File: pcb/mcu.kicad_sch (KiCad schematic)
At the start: 35 parts, among them J1 XF2M-1415-1A, SW1 EVQ-Q2B02W, SW2 EVQ-Q2B02W, U1 ESP32-S3-WROOM-1-N8R2

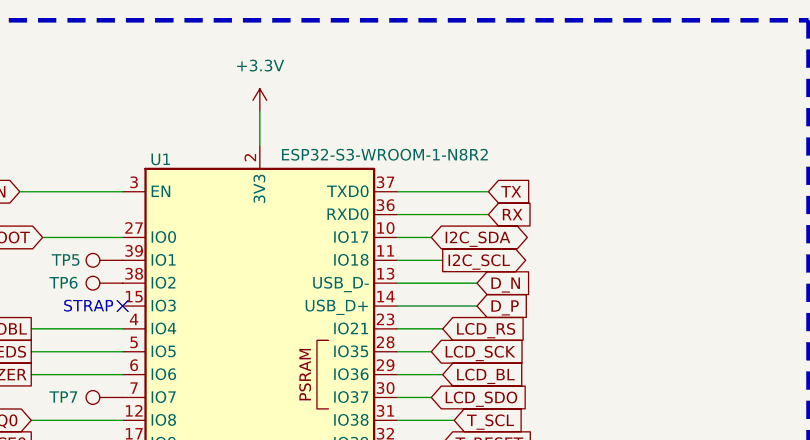
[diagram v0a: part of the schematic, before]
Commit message: Minor updates to ESP part number/footprint
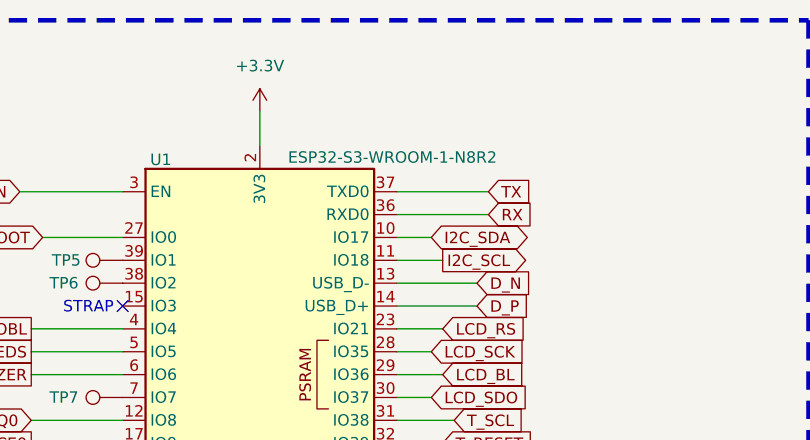
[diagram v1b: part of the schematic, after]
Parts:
- U1: symbol RF_Module:ESP32-S3-WROOM-1 -> CRG Makes:ESP32-S3-WROOM-1-N8R2
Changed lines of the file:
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@@
 	)
 	(symbol
-		(lib_id "RF_Module:ESP32-S3-WROOM-1")
+		(lib_id "CRG Makes:ESP32-S3-WROOM-1-N8R2")
 		(at 73.66 58.42 0)
 		(unit 1)
@@
 		)
 		(property "Value" "ESP32-S3-WROOM-1-N8R2"
-			(at 75.946 31.496 0)
+			(at 88.392 31.75 0)
 			(effects
 				(font
 					(size 1.27 1.27)
 				)
-				(justify left)
 			)
 		)
 		(property "Footprint" "CRG Makes:ESP32-S3-WROOM-1-N8R2"
-			(at 73.66 55.88 0)
+			(at 73.66 97.536 0)
 			(effects
 				(font
@@
 		)
 		(property "Datasheet" "https://www.espressif.com/sites/default/files/documentation/esp32-s3-wroom-1_wroom-1u_datasheet_en.pdf"
-			(at 73.66 58.42 0)
+			(at 73.66 103.886 0)
 			(effects
 				(font
@@
 			)
 		)
-		(property "Description" "RF Module, ESP32-S3 SoC"
-			(at 73.66 58.42 0)
+		(property "Description" "RF Module, ESP32-S3 SoC, Wi-Fi 802.11b/g/n, Bluetooth, BLE, 32-bit, 3.3V, onboard antenna, SMD"
+			(at 73.66 101.854 0)
 			(effects
 				(font
@@
 		)
 		(property "Mouser" "356-ESP32-S3WRM1N8R2"
-			(at 73.66 58.42 0)
+			(at 73.66 110.49 0)
 			(effects
 				(font
@@
 		)
 		(property "Digikey" "5407-ESP32-S3-WROOM-1-N8R2-ND"
-			(at 73.66 58.42 0)
+			(at 73.66 108.204 0)
 			(effects
 				(font
@@
 		)
 		(property "LCSC" "C2913204"
-			(at 73.66 58.42 0)
+			(at 73.66 112.776 0)
 			(effects
 				(font
